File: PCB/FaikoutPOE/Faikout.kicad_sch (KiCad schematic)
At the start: 84 parts, among them J1 RJ45_LED, J2 S21, J5 Reset, J7 TC2030-USB-NL-DS, M3 Ag97012-FL, P1 Square, Q1 BSS138PS, U1 KSZ8851SNL, U2 ESP32-S3-MINI-1, U3 TCMT1100, U4 TPS62933, U5 TCMT1100, Y1 Crystal_GND24

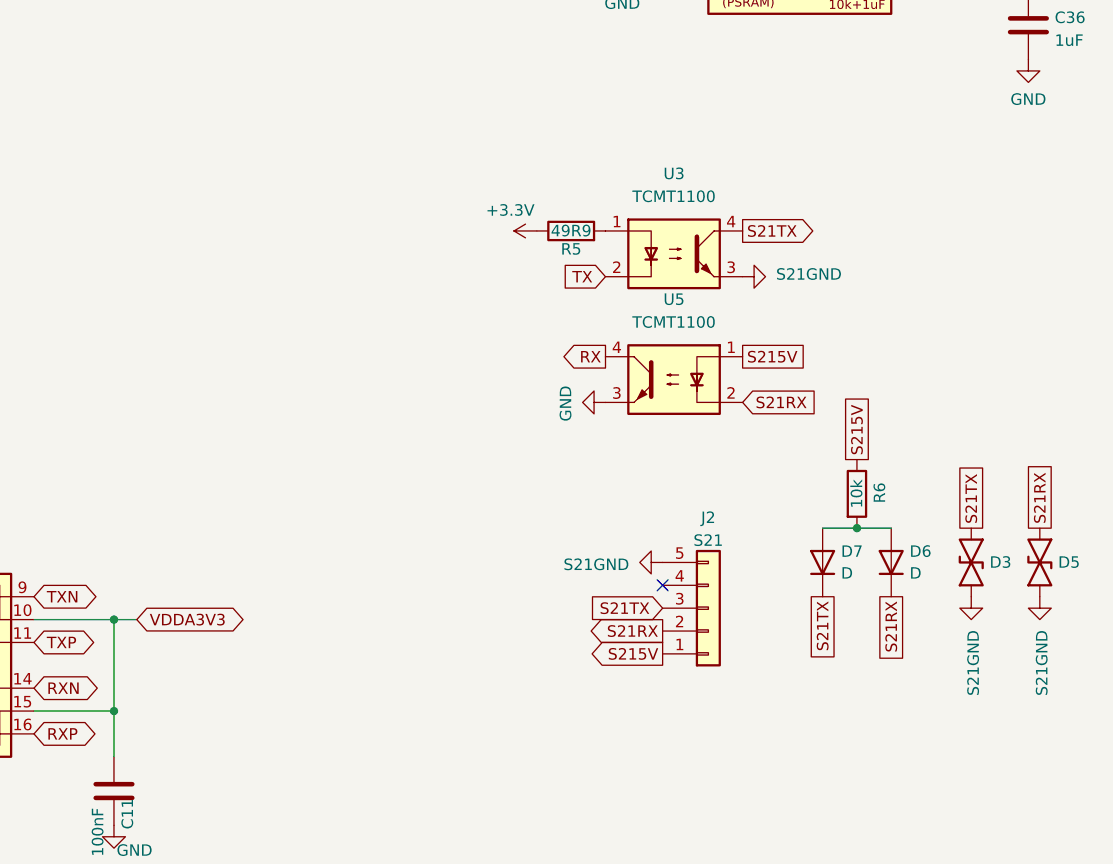
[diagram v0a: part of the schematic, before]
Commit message: PoE layout, not tracked yet
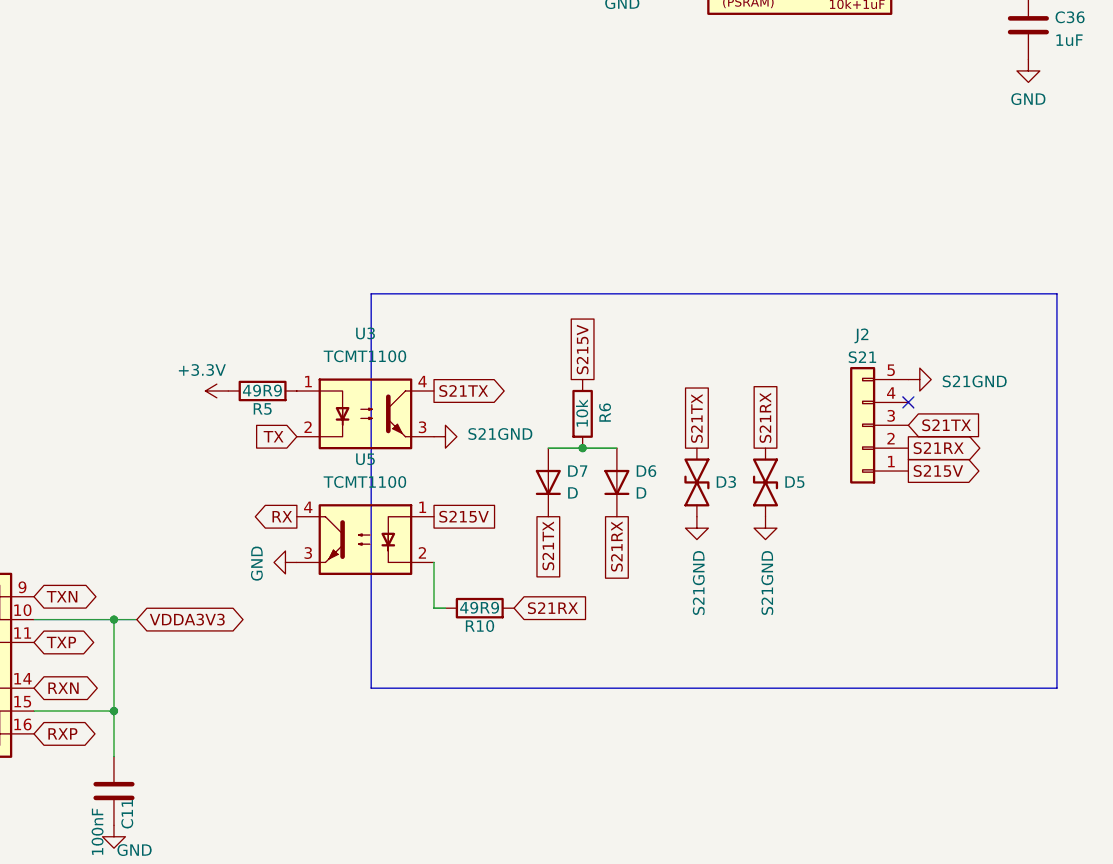
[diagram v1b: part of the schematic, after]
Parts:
- added R10: 49R9, RevK:R_0201, symbol Device:R
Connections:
- net S21RX: now also R10.2; no longer U5.2
- new net: R10.1, U5.2
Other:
- moved on the sheet: D3, D5, D6, D7, J2, R5, R6, U3, U5

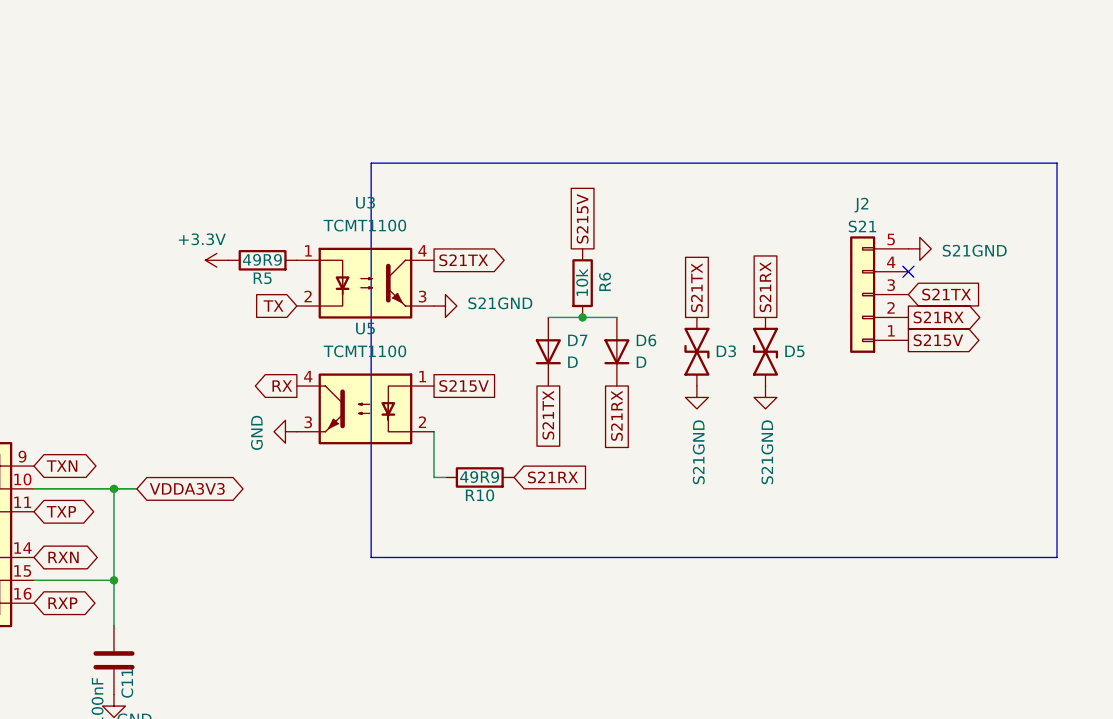
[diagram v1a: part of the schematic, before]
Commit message: Tweaks
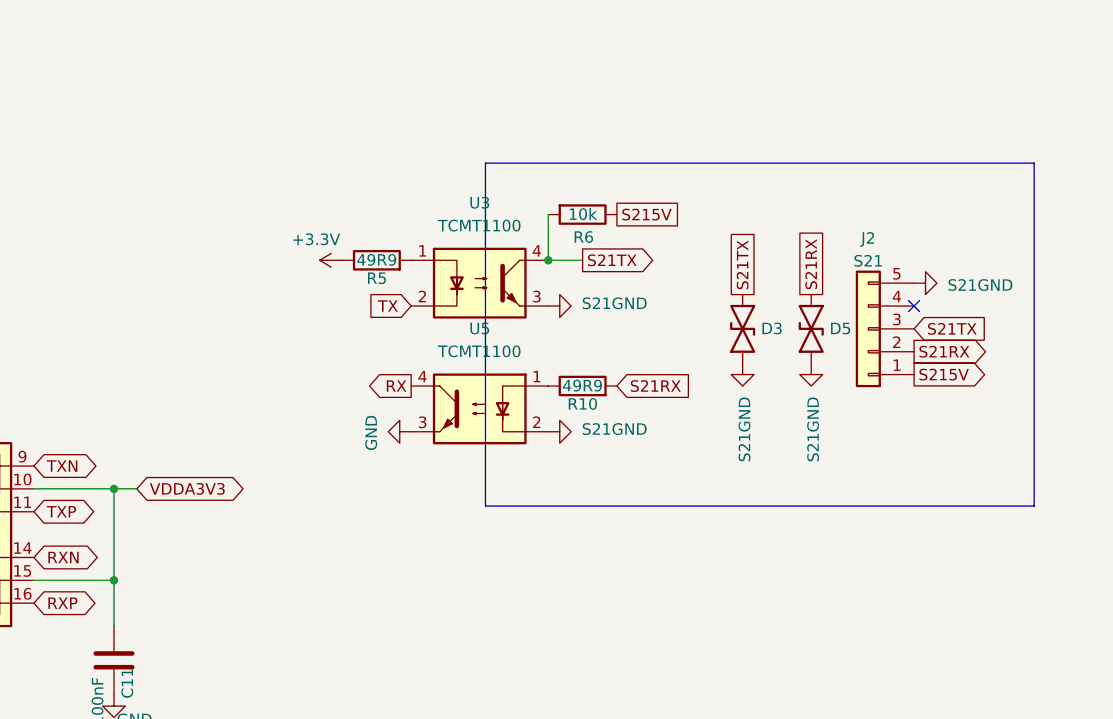
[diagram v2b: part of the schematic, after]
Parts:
- removed D6, D7: D, RevK:D_0402, symbol Device:D
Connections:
- net S215V: no longer U5.1
- net S21GND: now also U5.2
- net S21TX: now also R6.2
- net at R10.1: now also U5.1; no longer U5.2
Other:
- moved on the sheet: D3, D5, J2, R10, R5, R6, U3, U5
